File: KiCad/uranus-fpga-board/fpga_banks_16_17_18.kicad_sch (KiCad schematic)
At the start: 1 part, among them U20 XC7K325T-3FFG900E

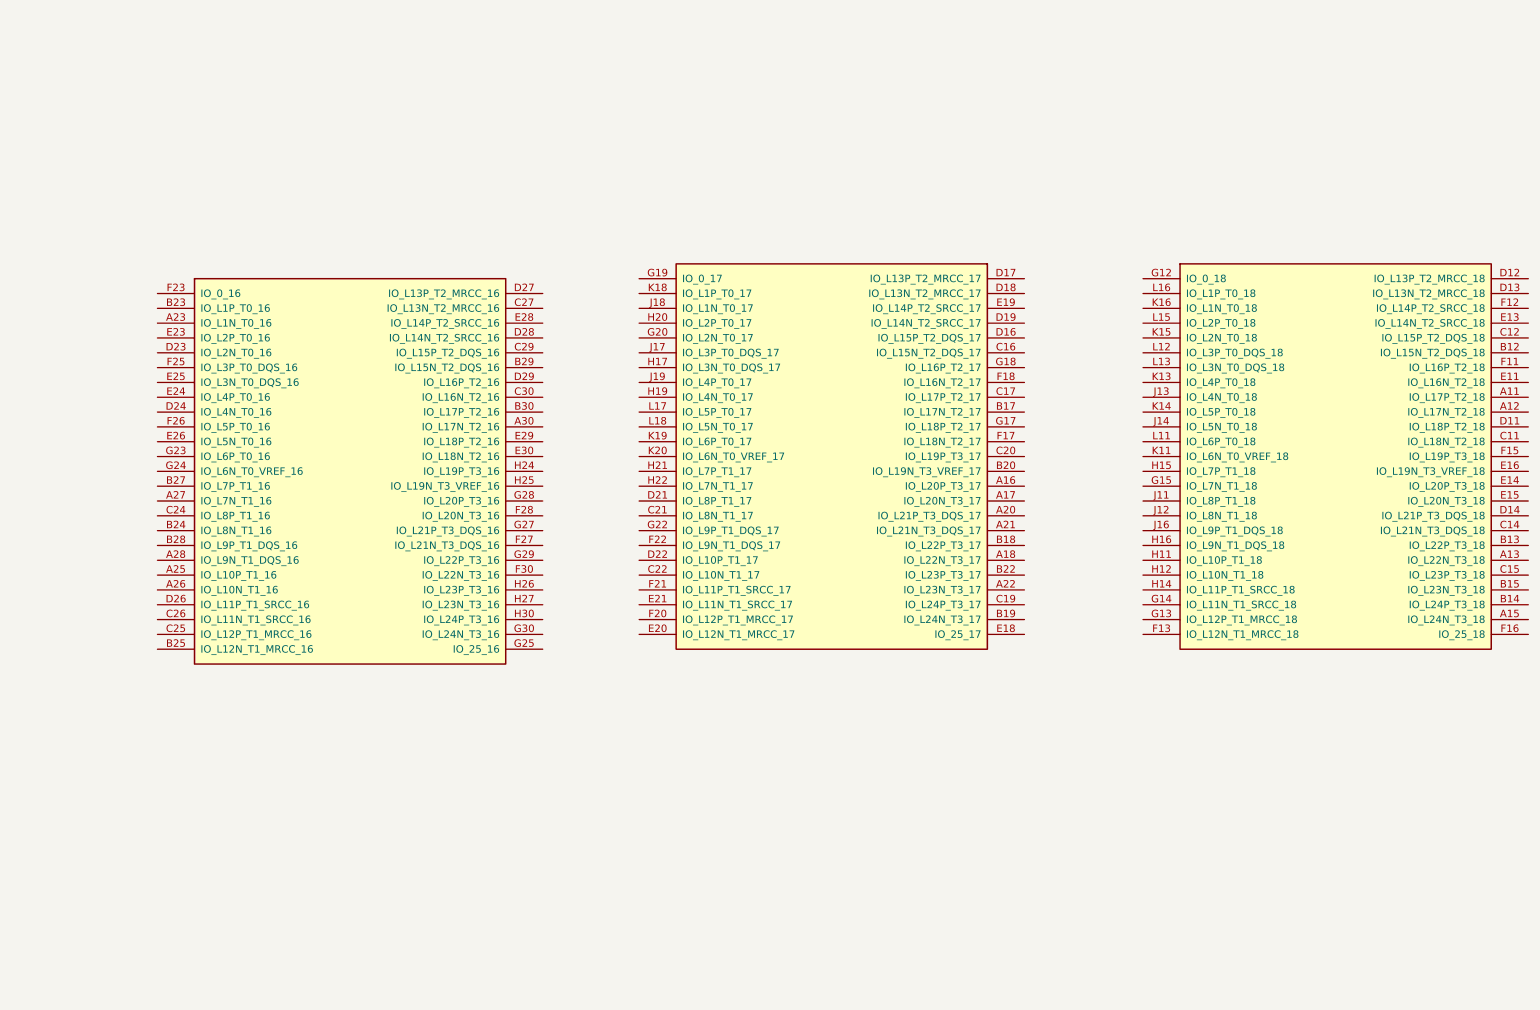
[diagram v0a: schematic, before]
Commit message: Big things have mostly happened in schematic quality
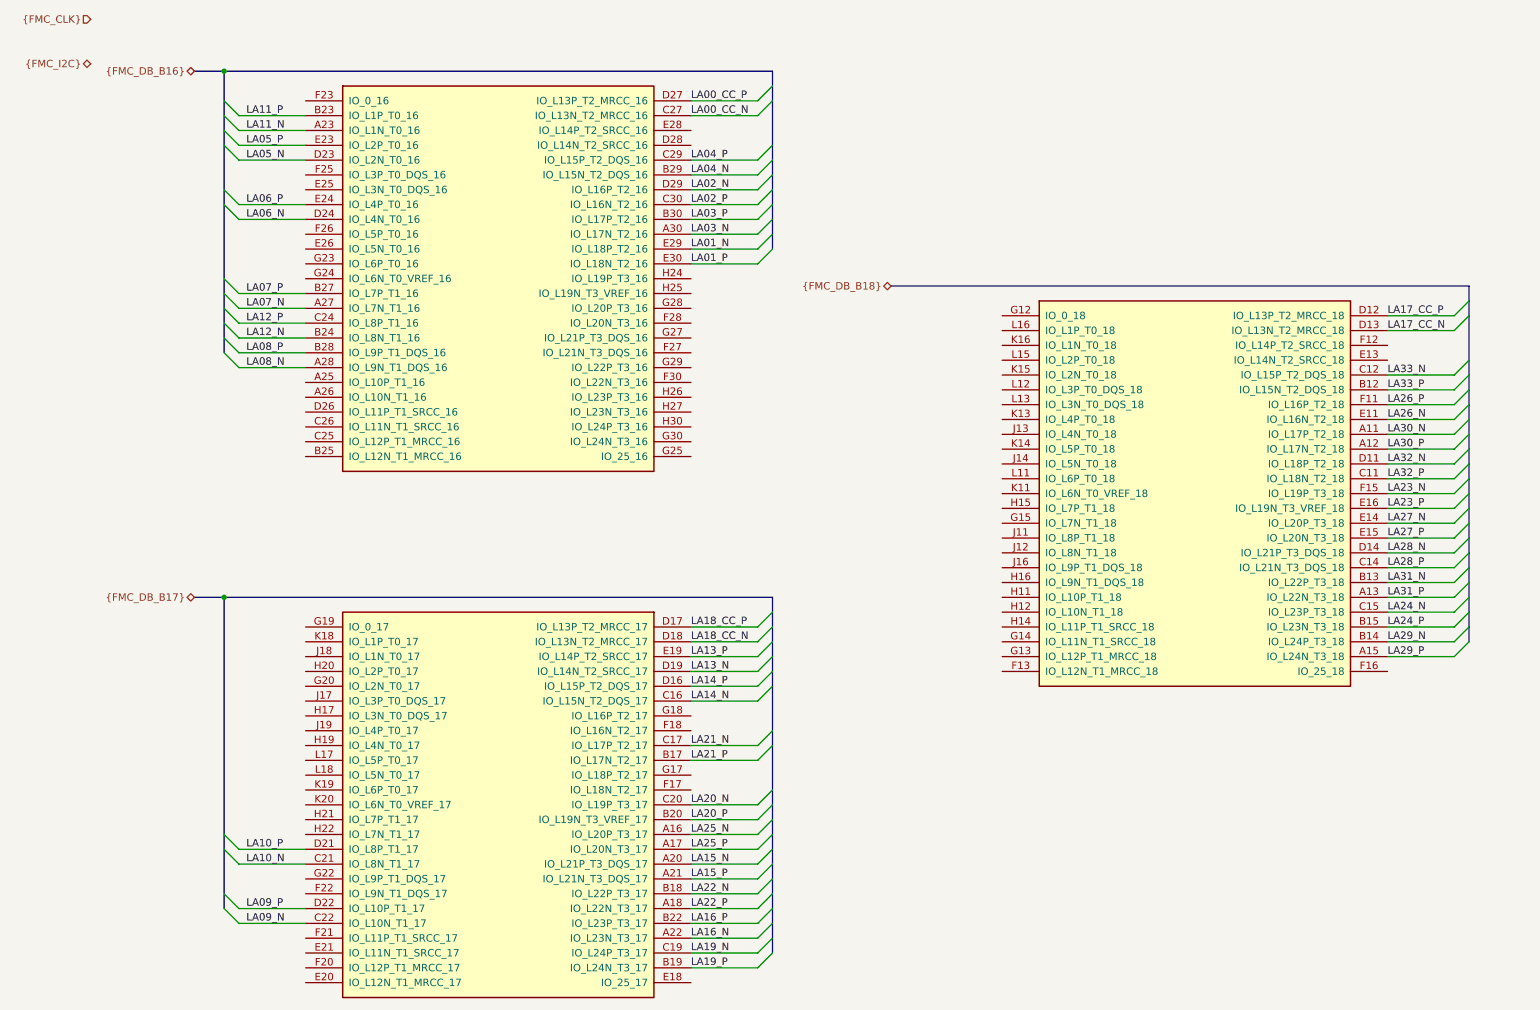
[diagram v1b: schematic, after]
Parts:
- renumbered U20 to U12
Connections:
- net LA25_N: now reaches U12.A16 (IO_L20P_T3_17)
- net LA25_P: now reaches U12.A17 (IO_L20N_T3_17)
- net LA22_P: now reaches U12.A18 (IO_L22N_T3_17)
- net LA15_N: now reaches U12.A20 (IO_L21P_T3_DQS_17)
- net LA15_P: now reaches U12.A21 (IO_L21N_T3_DQS_17)
- net LA16_N: now reaches U12.A22 (IO_L23N_T3_17)
- net LA21_P: now reaches U12.B17 (IO_L17N_T2_17)
- net LA22_N: now reaches U12.B18 (IO_L22P_T3_17)
- net LA19_P: now reaches U12.B19 (IO_L24N_T3_17)
- net LA20_P: now reaches U12.B20 (IO_L19N_T3_VREF_17)
- net LA16_P: now reaches U12.B22 (IO_L23P_T3_17)
- net LA14_N: now reaches U12.C16 (IO_L15N_T2_DQS_17)
- net LA21_N: now reaches U12.C17 (IO_L17P_T2_17)
- net LA19_N: now reaches U12.C19 (IO_L24P_T3_17)
- net LA20_N: now reaches U12.C20 (IO_L19P_T3_17)
- net LA10_N: now reaches U12.C21 (IO_L8N_T1_17)
- net LA09_N: now reaches U12.C22 (IO_L10N_T1_17)
- net LA14_P: now reaches U12.D16 (IO_L15P_T2_DQS_17)
- net LA18_CC_P: now reaches U12.D17 (IO_L13P_T2_MRCC_17)
- net LA18_CC_N: now reaches U12.D18 (IO_L13N_T2_MRCC_17)
- net LA13_N: now reaches U12.D19 (IO_L14N_T2_SRCC_17)
- net LA10_P: now reaches U12.D21 (IO_L8P_T1_17)
- net LA09_P: now reaches U12.D22 (IO_L10P_T1_17)
- net LA13_P: now reaches U12.E19 (IO_L14P_T2_SRCC_17)
- net LA30_N: now reaches U12.A11 (IO_L17P_T2_18)
- net LA30_P: now reaches U12.A12 (IO_L17N_T2_18)
- net LA31_P: now reaches U12.A13 (IO_L22N_T3_18)
- net LA29_P: now reaches U12.A15 (IO_L24N_T3_18)
- net LA33_P: now reaches U12.B12 (IO_L15N_T2_DQS_18)
- net LA31_N: now reaches U12.B13 (IO_L22P_T3_18)
- net LA29_N: now reaches U12.B14 (IO_L24P_T3_18)
- net LA24_P: now reaches U12.B15 (IO_L23N_T3_18)
- net LA32_P: now reaches U12.C11 (IO_L18N_T2_18)
- net LA33_N: now reaches U12.C12 (IO_L15P_T2_DQS_18)
- net LA28_P: now reaches U12.C14 (IO_L21N_T3_DQS_18)
- net LA24_N: now reaches U12.C15 (IO_L23P_T3_18)
- net LA32_N: now reaches U12.D11 (IO_L18P_T2_18)
- net LA17_CC_P: now reaches U12.D12 (IO_L13P_T2_MRCC_18)
- net LA17_CC_N: now reaches U12.D13 (IO_L13N_T2_MRCC_18)
- net LA28_N: now reaches U12.D14 (IO_L21P_T3_DQS_18)
- net LA26_N: now reaches U12.E11 (IO_L16N_T2_18)
- net LA27_N: now reaches U12.E14 (IO_L20P_T3_18)
- net LA27_P: now reaches U12.E15 (IO_L20N_T3_18)
- net LA23_P: now reaches U12.E16 (IO_L19N_T3_VREF_18)
- net LA26_P: now reaches U12.F11 (IO_L16P_T2_18)
- net LA23_N: now reaches U12.F15 (IO_L19P_T3_18)
- net LA11_N: now reaches U12.A23 (IO_L1N_T0_16)
- net LA07_N: now reaches U12.A27 (IO_L7N_T1_16)
- net LA08_N: now reaches U12.A28 (IO_L9N_T1_DQS_16)
- net LA03_N: now reaches U12.A30 (IO_L17N_T2_16)
- net LA11_P: now reaches U12.B23 (IO_L1P_T0_16)
- net LA12_N: now reaches U12.B24 (IO_L8N_T1_16)
- net LA07_P: now reaches U12.B27 (IO_L7P_T1_16)
- net LA08_P: now reaches U12.B28 (IO_L9P_T1_DQS_16)
- net LA04_N: now reaches U12.B29 (IO_L15N_T2_DQS_16)
- net LA03_P: now reaches U12.B30 (IO_L17P_T2_16)
- net LA12_P: now reaches U12.C24 (IO_L8P_T1_16)
- net LA00_CC_N: now reaches U12.C27 (IO_L13N_T2_MRCC_16)
- net LA04_P: now reaches U12.C29 (IO_L15P_T2_DQS_16)
- net LA02_P: now reaches U12.C30 (IO_L16N_T2_16)
- net LA05_N: now reaches U12.D23 (IO_L2N_T0_16)
- net LA06_N: now reaches U12.D24 (IO_L4N_T0_16)
- net LA00_CC_P: now reaches U12.D27 (IO_L13P_T2_MRCC_16)
- net LA02_N: now reaches U12.D29 (IO_L16P_T2_16)
- net LA05_P: now reaches U12.E23 (IO_L2P_T0_16)
- net LA06_P: now reaches U12.E24 (IO_L4P_T0_16)
- net LA01_N: now reaches U12.E29 (IO_L18P_T2_16)
- net LA01_P: now reaches U12.E30 (IO_L18N_T2_16)
